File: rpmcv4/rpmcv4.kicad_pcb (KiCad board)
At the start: 2 copper layers, 88.3 x 97.8 mm, 31 parts, among them J1 RPi_GPIO, P1 CONN_02X25, P2 CONN_02X25, U1 74LS373, U2 74LS373, U3 74LS245, U7 74LS245, U8 74LS245

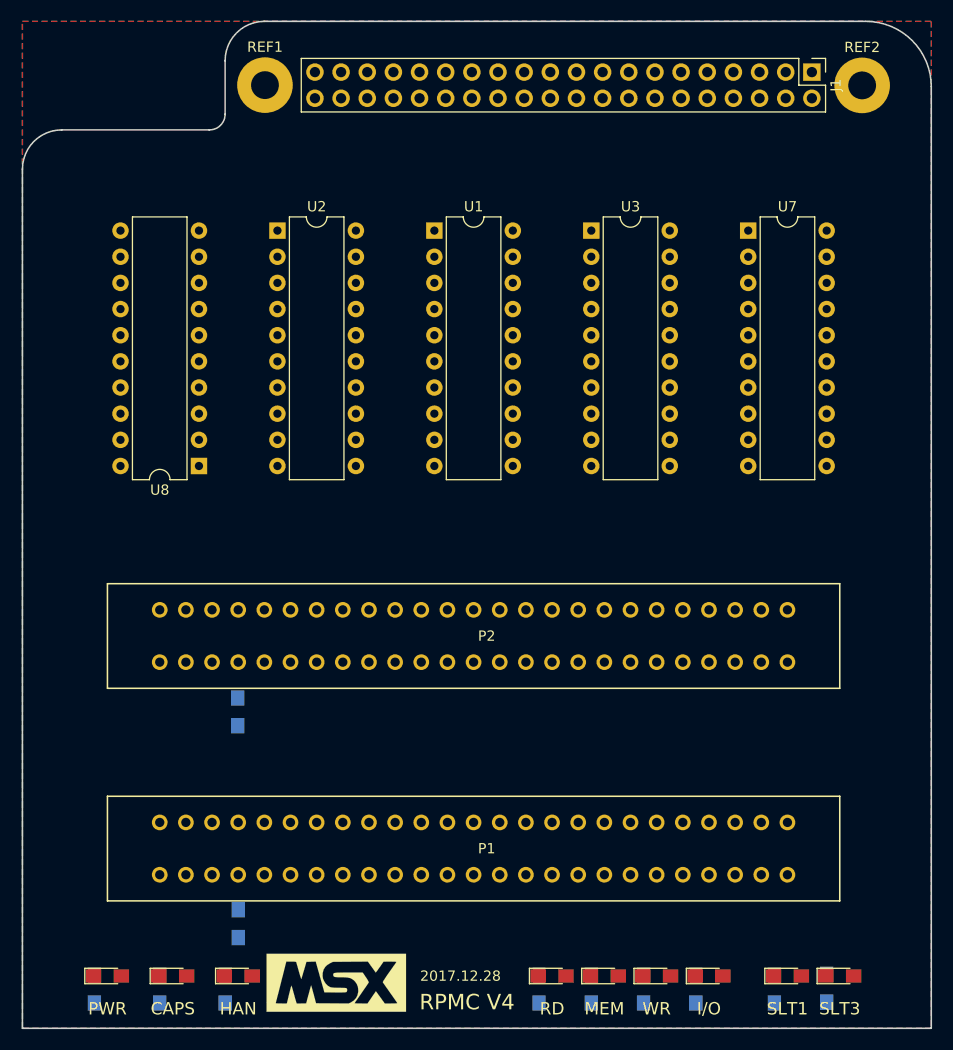
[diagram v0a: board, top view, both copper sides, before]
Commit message: small improvement
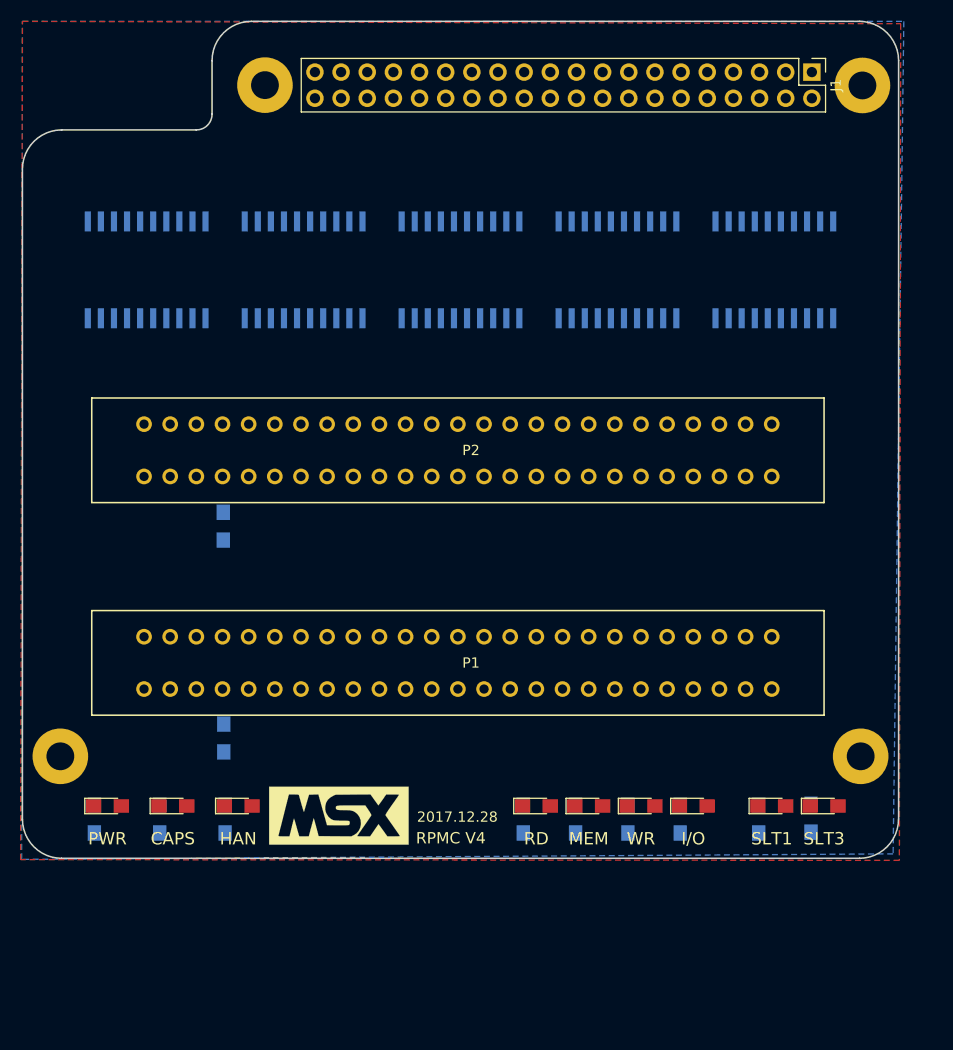
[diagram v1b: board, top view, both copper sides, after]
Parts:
- added REF3: MountingHole_2.7mm_Pad, Mounting_Holes:MountingHole_2.7mm_Pad, F.Cu at (132.6, 122.2)
- added REF4: MountingHole_2.7mm_Pad, Mounting_Holes:MountingHole_2.7mm_Pad, F.Cu at (210.3, 122.2)
- U1, U2, U3, U7, U8: footprint Housings_DIP:DIP-20_W7.62mm -> Housings_SOIC:SOIC-20_7.5x12.8mm_Pitch1.27mm; moved to B.Cu
- moved U8 19.7 mm to (141.0, 74.9), turned to 270 degrees
- moved P1 18.1 mm to (172.5, 113.1)
- moved P2 18.1 mm to (172.5, 92.5)
- moved R11 18.1 mm to (148.4, 99.8)
- moved R10 18.1 mm to (148.5, 120.4)
- moved D1 16.6 mm to (206.8, 127.0)
- moved D2 16.6 mm to (201.7, 127.0)
- moved D3 16.6 mm to (194.1, 127.0)
- moved D4 16.6 mm to (189.0, 127.0)
- moved D5 16.6 mm to (183.9, 127.0)
- moved D6 16.6 mm to (178.8, 127.0)
- moved R1 16.6 mm to (205.5, 128.2)
- moved R2 16.6 mm to (200.4, 128.3)
- moved R3 16.6 mm to (192.8, 128.3)
- moved R4 16.6 mm to (187.7, 128.3)
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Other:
- board size 88.3 x 97.8 mm -> 85.1 x 81.3 mm
